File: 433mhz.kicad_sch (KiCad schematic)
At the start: 4 parts, among them J4 Conn_Coaxial, U3 RFM96W-433S2

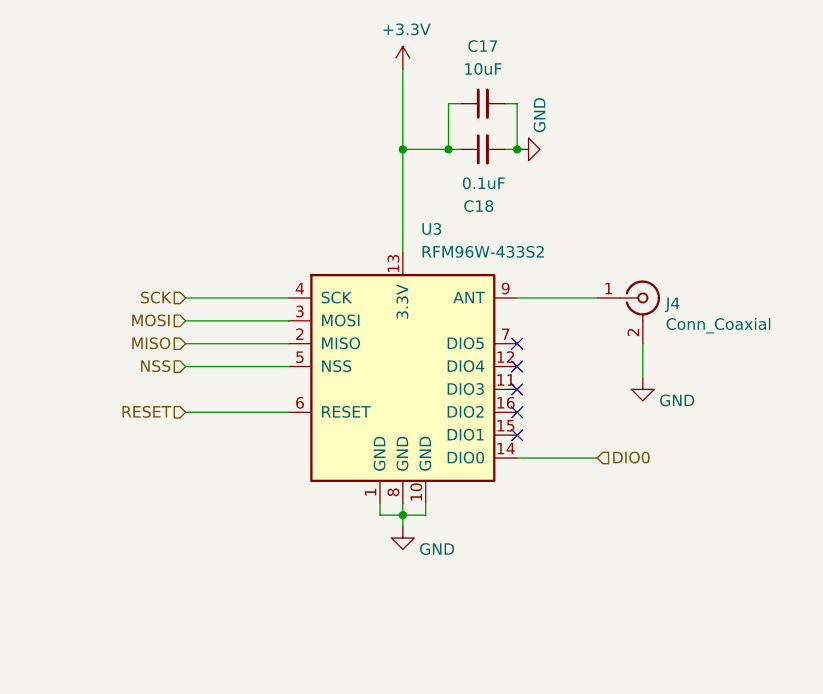
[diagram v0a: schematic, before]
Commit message: New Template Update
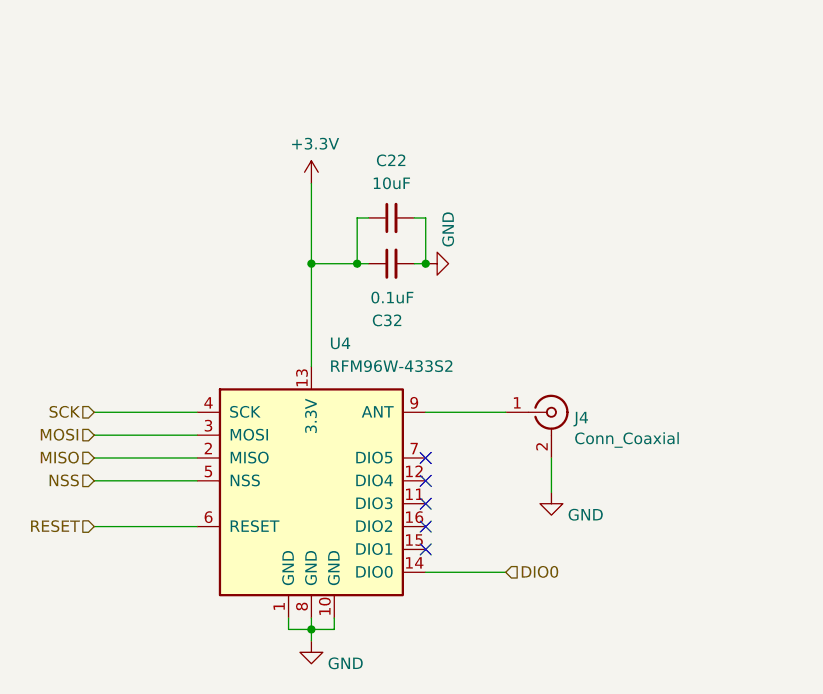
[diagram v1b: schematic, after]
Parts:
- removed C17: 10uF, Capacitor_SMD:C_0603_1608Metric, symbol Device:C_Small
- removed C18: 0.1uF, Capacitor_SMD:C_0603_1608Metric, symbol Device:C_Small
- removed U3: RFM96W-433S2, RF_Module:HOPERF_RFM9XW_SMD, symbol RF_Module:RFM96W-433S2
- added C22: 10uF, Capacitor_SMD:C_0402_1005Metric, symbol Device:C_Small
- added C32: 0.1uF, Capacitor_SMD:C_0402_1005Metric, symbol Device:C_Small
- added U4: RFM96W-433S2, RF_Module:HOPERF_RFM9XW_SMD, symbol RF_Module:RFM96W-433S2
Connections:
- net +3V3: now also C22.1, C32.1, U4.13 (3.3V)
- net DIO0: now also U4.14 (DIO0)
- net GND: now also C22.2, C32.2, U4.1 (GND), U4.10 (GND), U4.8 (GND)
- net MISO: now also U4.2 (MISO)
- net MOSI: now also U4.3 (MOSI)
- net NSS: now also U4.5 (NSS)
- net RESET: now also U4.6 (RESET)
- net SCK: now also U4.4 (SCK)
- net at J4.1 (In): now also U4.9 (ANT)
